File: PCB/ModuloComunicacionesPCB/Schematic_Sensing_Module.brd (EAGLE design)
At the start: 74 parts, among them Q1 CSM-7X-DU

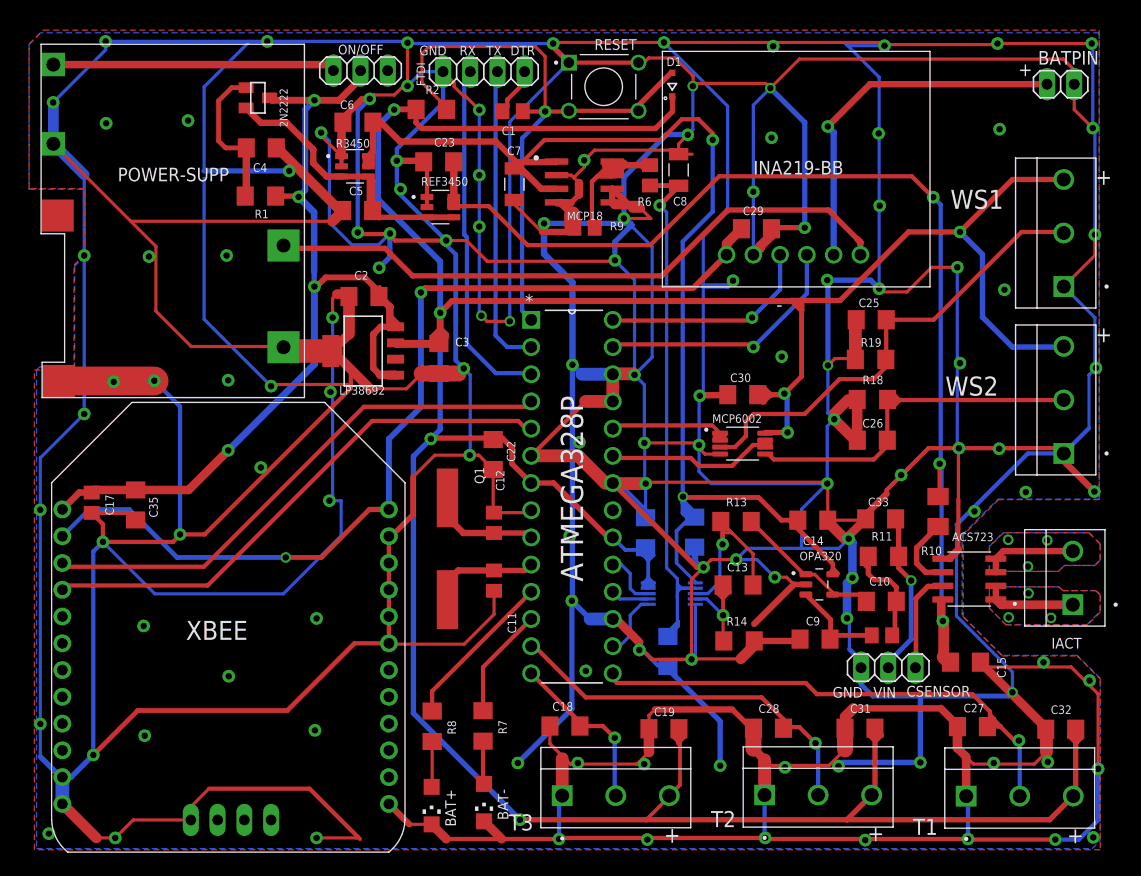
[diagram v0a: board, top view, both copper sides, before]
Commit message: transmisor terminado
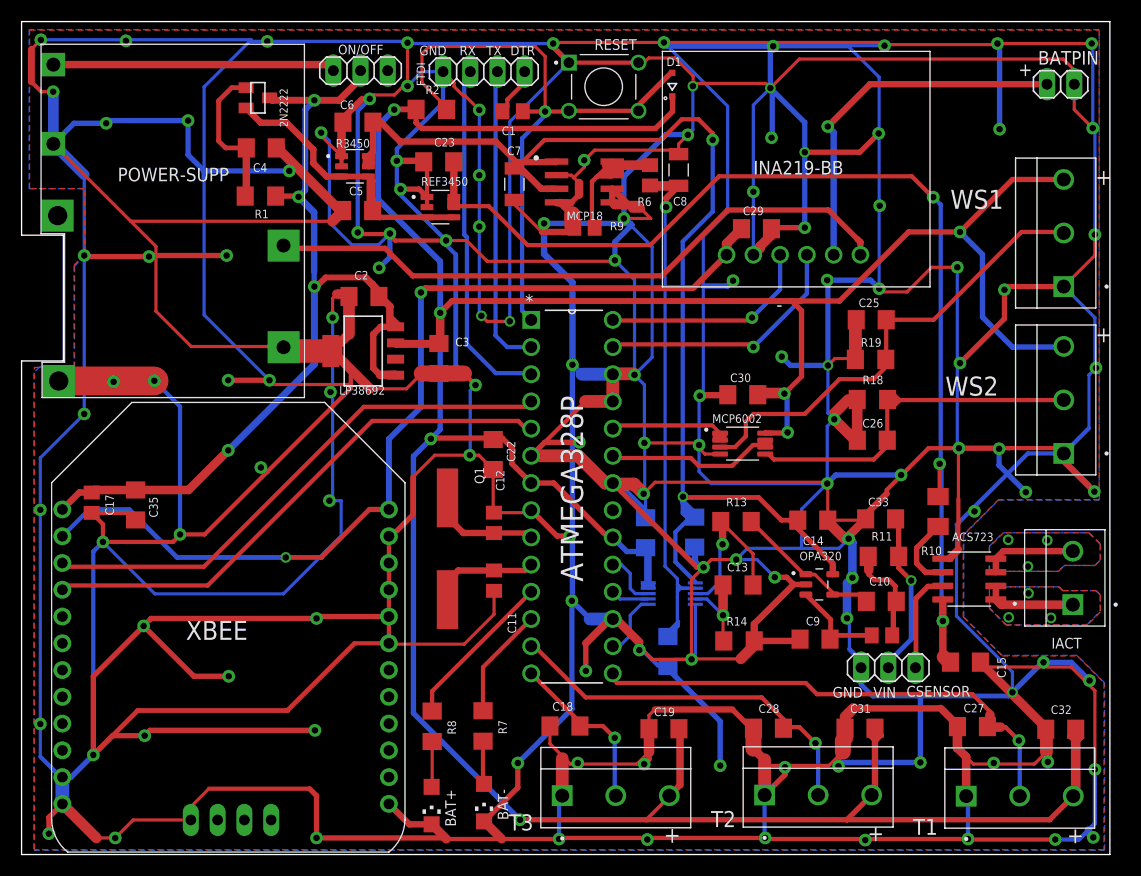
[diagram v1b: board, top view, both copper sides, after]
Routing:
- net GND: track 1706.7 -> 1959.7 mm, vias 124 -> 126
- net VLP5: track 345.5 -> 324.0 mm
- net VOMCP18: track 23.8 -> 19.0 mm
- net IN-: track 13.2 -> 8.48 mm
- net VREF18: track 56.1 -> 53.3 mm
- net IN+: track 18.0 -> 15.5 mm
- net VSUPPLY: track 90.9 -> 89.2 mm
- net DATAT1: track 48.8 -> 47.2 mm
- net N$14: track 10.9 -> 9.43 mm
- net VREF5: track 121.2 -> 119.8 mm
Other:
- board outline added: 101.7 x 77.8 mm
